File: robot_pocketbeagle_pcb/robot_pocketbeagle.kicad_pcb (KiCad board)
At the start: 2 copper layers, 75 x 100 mm, 104 parts, among them J1 QMC5883L, J10 driver_dvr8833, J12 IN_DVR8833, J13 9V_DC_DC, J14 servo_x_y, J15 shr05, J16 5V_DC_DC, J17 Conn_GND, J18 Conn_5V, J19 Conn_pwm_out_b, J2 USB_A, J20 Conn_pwm_out_a, J21 Conn_P2_3.3V, J29 Conn_AIN_4.096_3.3_1.8V, J3 UART0, J30 Conn_5V, J31 Conn_GPI028_34, J4 P1, J5 MPU6050, J6 ADS1115, J7 P2, J8 Conn_i2c2, J9 OUT_DVR8833, Q1 BC847, Q2 BC847, Q3 QM6015D, Q4 BC847, Q5 BC847, Q6 QM6015D, Q7 QM6015D, U1 PC817, U2 PC817, U3 74HC00, U4 LM358, U5 L7805_REZERV

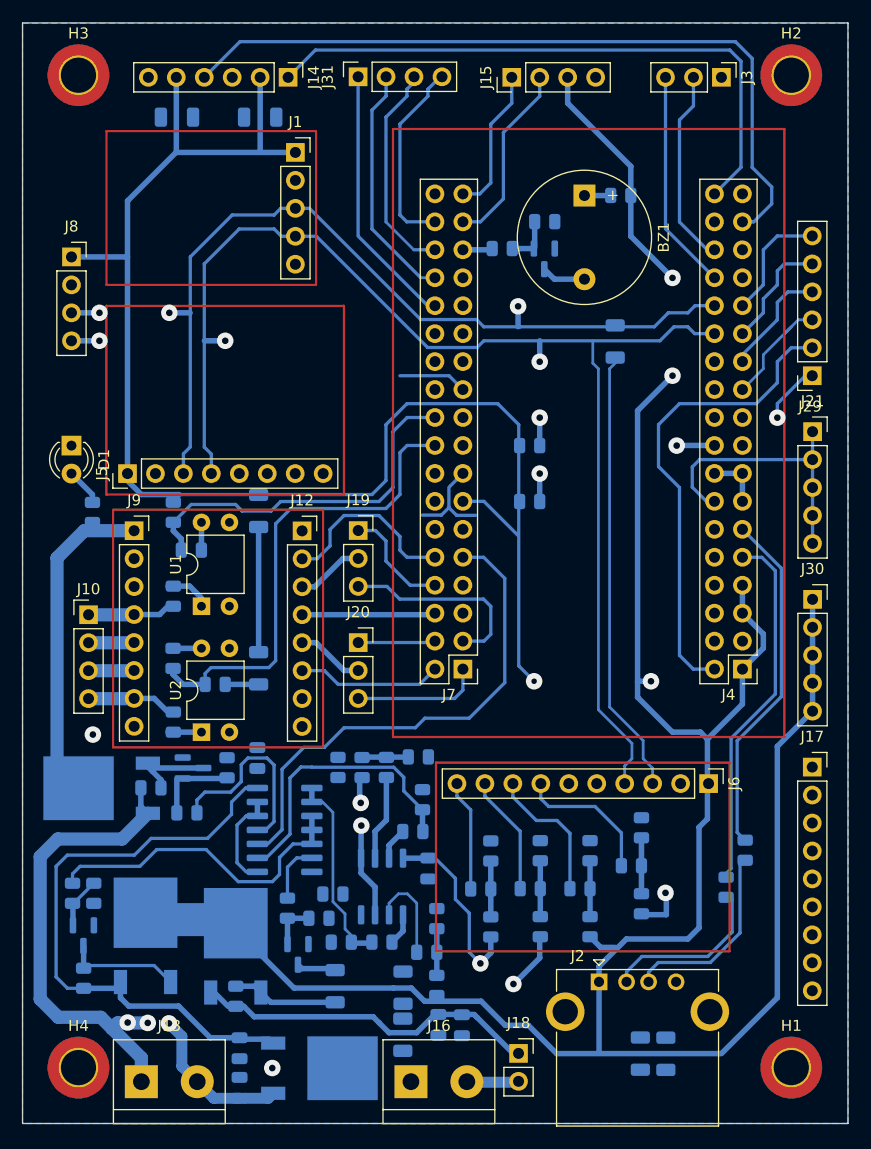
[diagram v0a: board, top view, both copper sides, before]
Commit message: board debugging 1
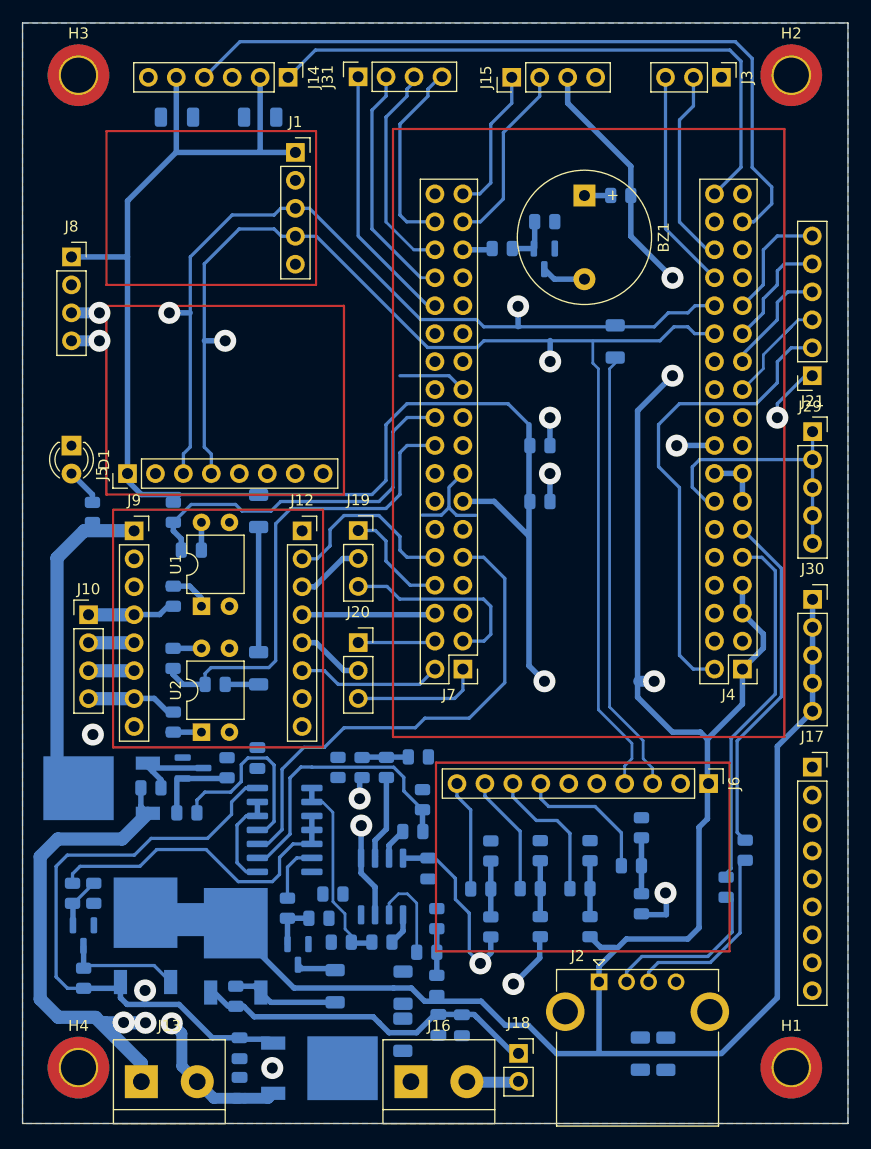
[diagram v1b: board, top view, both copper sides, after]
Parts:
- moved R38 0.93 mm to (148.6, 65.4)
- moved R39 0.93 mm to (148.6, 70.5)
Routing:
- net P1_SYS_VIN: track 373.1 -> 375.1 mm
- net AUX_5V_OUT: track 55.5 -> 56.7 mm, vias 0 -> 1
- net 9V_DRIVER_DC_DC_IN: track 52.8 -> 51.8 mm
